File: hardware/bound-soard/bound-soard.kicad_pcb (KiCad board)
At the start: 2 copper layers, 17 parts, among them J1 Signal_Input, J2 Conn_01x02_Female, J3 Conn_01x02_Male, J4 Conn_01x02_Female, J5 Supply, J6 Conn_01x02_Male, J7 Conn_01x02_Female, J8 Conn_01x02_Male, J9 Signal_Output

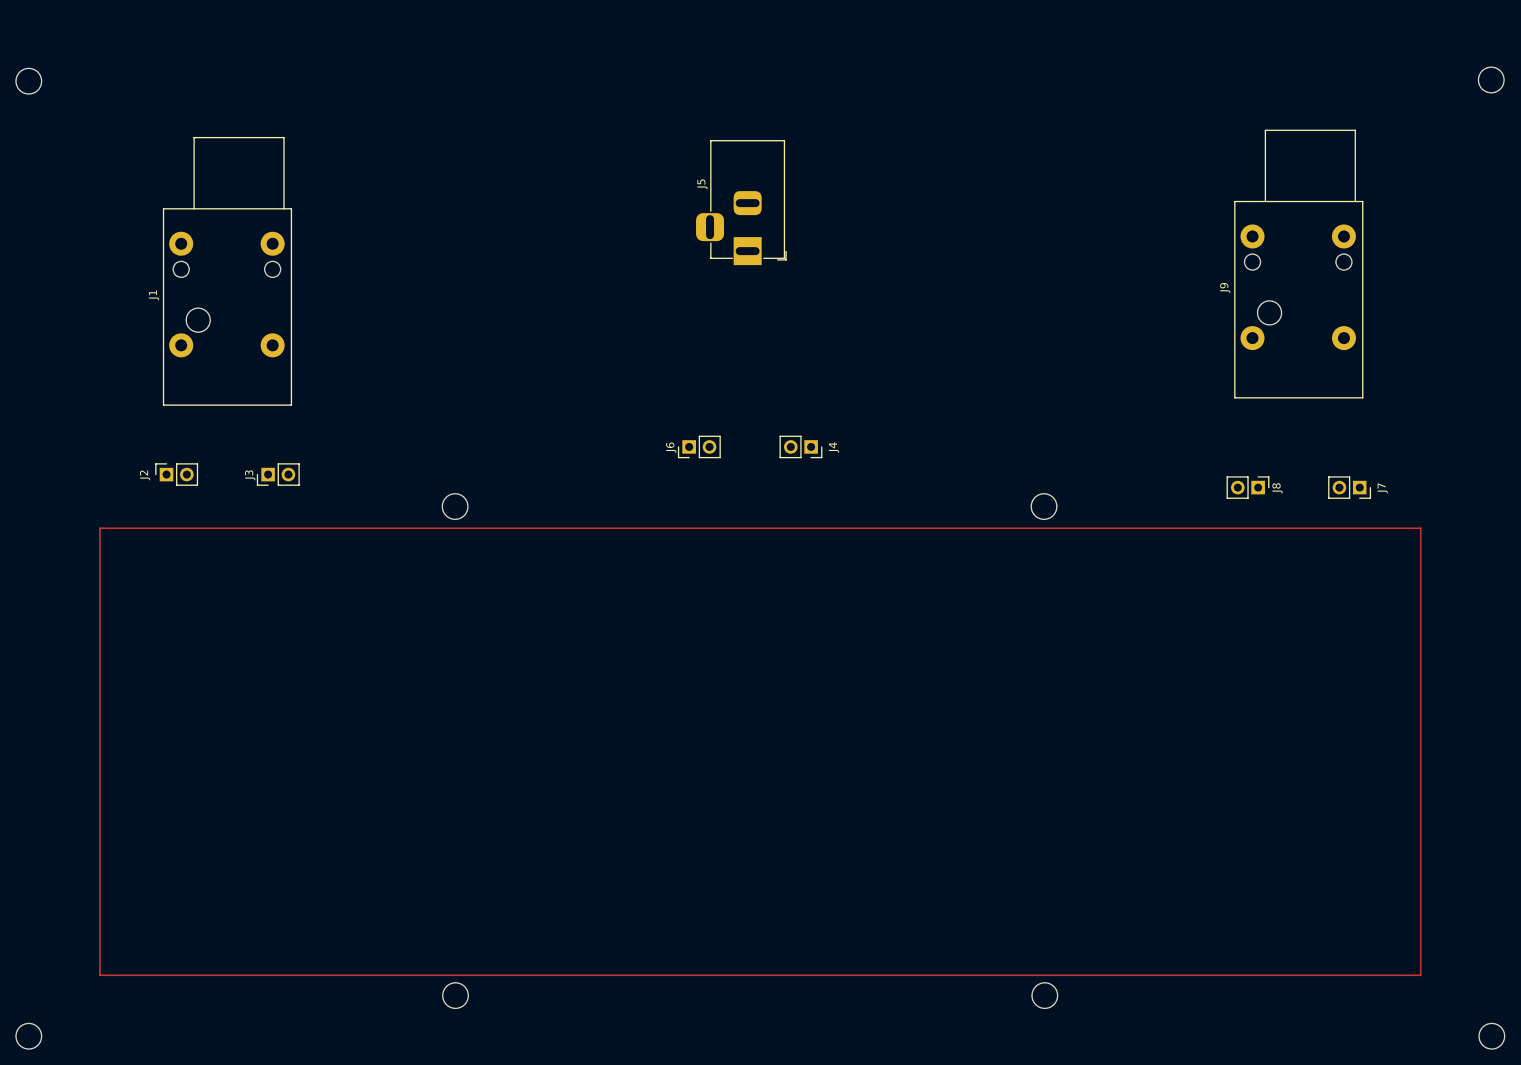
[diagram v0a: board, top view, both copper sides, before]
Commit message: probably final
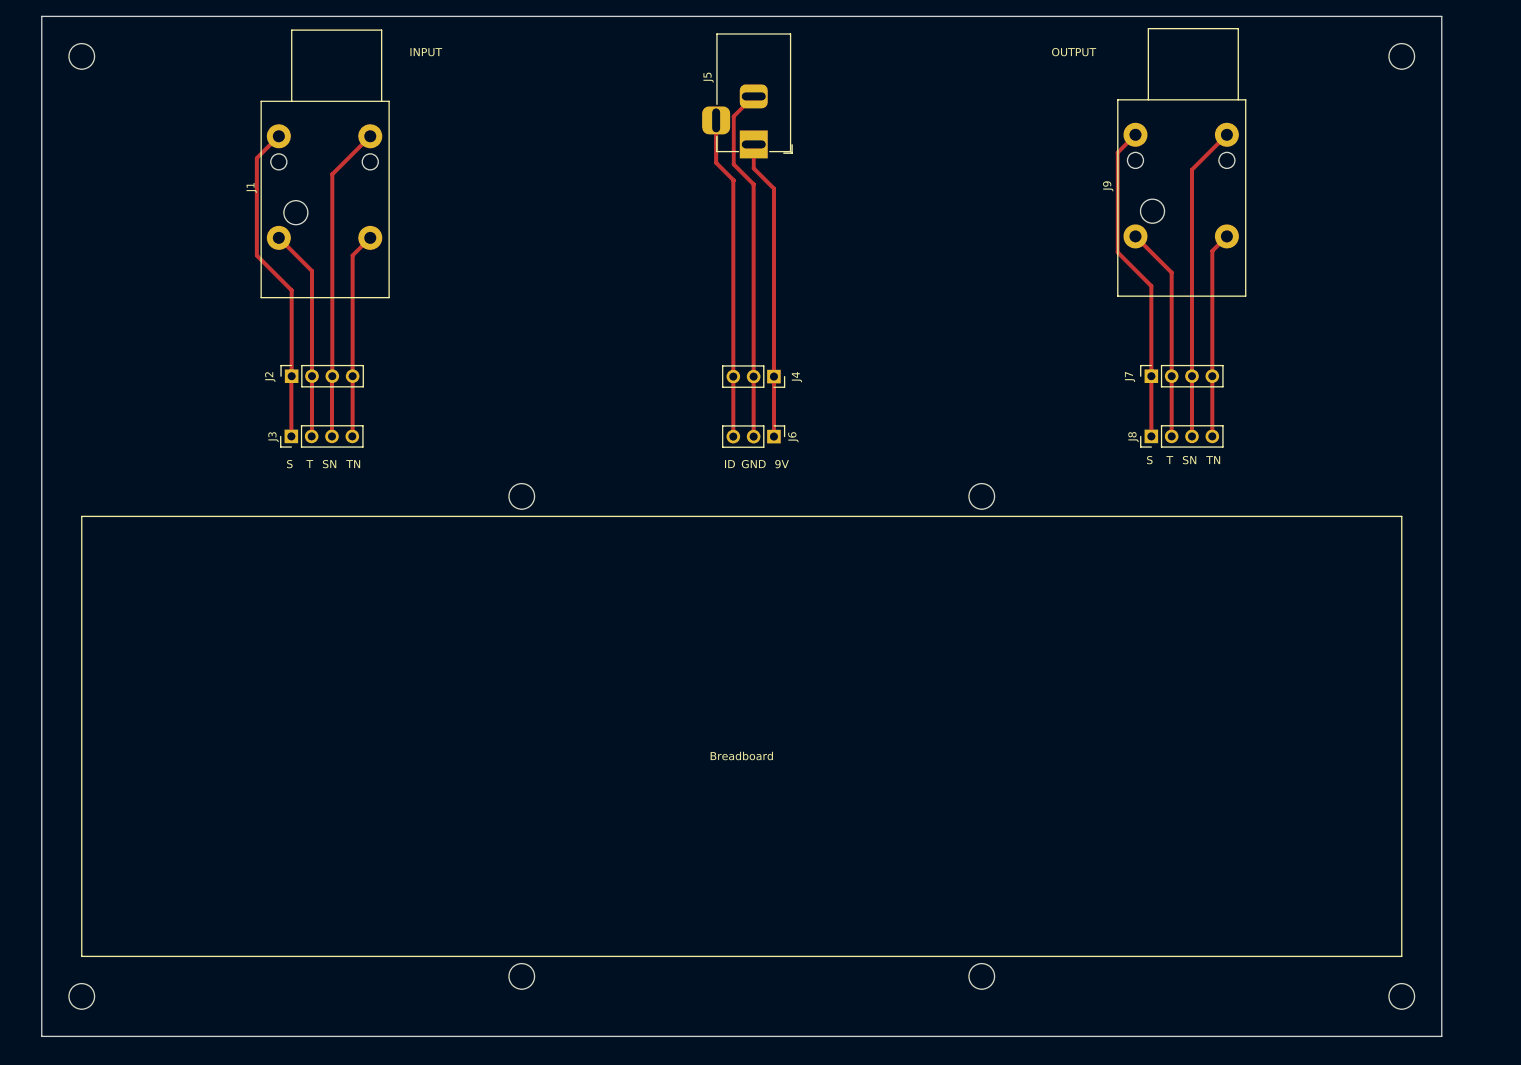
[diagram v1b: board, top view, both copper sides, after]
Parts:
- removed the REF** at (55.9, 38.1)
- removed the REF** at (238.7, 37.9)
- removed the REF** at (182.9, 152.4)
- removed the REF** at (238.8, 157.5)
- removed the REF** at (182.8, 91.3)
- removed the REF** at (55.9, 157.5)
- removed the REF** at (109.2, 152.4)
- removed the REF** at (109.2, 91.3)
- added REF**: MountingHole_3.2mm_M3_ISO14580, MountingHole:MountingHole_3.2mm_M3_ISO14580, F.Cu at (227.5, 152.5)
- added REF**: MountingHole_3.2mm_M3_ISO14580, MountingHole:MountingHole_3.2mm_M3_ISO14580, F.Cu at (117.5, 150.0)
- added REF**: MountingHole_3.2mm_M3_ISO14580, MountingHole:MountingHole_3.2mm_M3_ISO14580, F.Cu at (117.5, 90.0)
- added REF**: MountingHole_3.2mm_M3_ISO14580, MountingHole:MountingHole_3.2mm_M3_ISO14580, F.Cu at (62.5, 35.0)
- added REF**: MountingHole_3.2mm_M3_ISO14580, MountingHole:MountingHole_3.2mm_M3_ISO14580, F.Cu at (175.0, 90.0)
- added REF**: MountingHole_3.2mm_M3_ISO14580, MountingHole:MountingHole_3.2mm_M3_ISO14580, F.Cu at (62.5, 152.5)
- added REF**: MountingHole_3.2mm_M3_ISO14580, MountingHole:MountingHole_3.2mm_M3_ISO14580, F.Cu at (175.0, 150.0)
- added REF**: MountingHole_3.2mm_M3_ISO14580, MountingHole:MountingHole_3.2mm_M3_ISO14580, F.Cu at (227.5, 35.0)
- J1: value Signal_Input -> AudioJack2_Dual_Switch
- J2, J7: value Conn_01x02_Female -> Conn_01x04_Female; footprint Connector_PinSocket_2.54mm:PinSocket_1x02_P2.54mm_Vertical -> Connector_PinSocket_2.54mm:PinSocket_1x04_P2.54mm_Vertical
- J3, J8: value Conn_01x02_Male -> Conn_01x04_Male; footprint Connector_PinHeader_2.54mm:PinHeader_1x02_P2.54mm_Vertical -> Connector_PinHeader_2.54mm:PinHeader_1x04_P2.54mm_Vertical
- J4: value Conn_01x02_Female -> Conn_01x03_Female; footprint Connector_PinSocket_2.54mm:PinSocket_1x02_P2.54mm_Vertical -> Connector_PinSocket_2.54mm:PinSocket_1x03_P2.54mm_Vertical
- J5: value Supply -> 9V Supply
- J6: value Conn_01x02_Male -> Conn_01x03_Male; footprint Connector_PinHeader_2.54mm:PinHeader_1x02_P2.54mm_Vertical -> Connector_PinHeader_2.54mm:PinHeader_1x03_P2.54mm_Vertical
- J9: value Signal_Output -> AudioJack2_Dual_Switch
- moved J7 29.5 mm to (196.2, 75.0), turned to 90 degrees
- moved J2 19.9 mm to (88.7, 75.0)
- moved J9 19.4 mm to (194.2, 57.5)
- moved J1 18.2 mm to (87.1, 57.7)
- moved J8 14.8 mm to (196.2, 82.5), turned to 90 degrees
- moved J5 13.4 mm to (146.5, 46.0)
- moved J6 10.7 mm to (149.0, 82.5), turned to -90 degrees
- moved J4 9.95 mm to (149.0, 75.0)
- moved J3 5.58 mm to (88.7, 82.5)
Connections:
- J1 pad SN: (no net) -> Net-(J1-PadSN)
- J1 pad TN: (no net) -> Net-(J1-PadTN)
- J5 pad 3: (no net) -> Net-(J4-Pad3)
- J9 pad SN: (no net) -> Net-(J7-Pad3)
- J9 pad TN: (no net) -> Net-(J7-Pad4)
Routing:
- net Net-(J4-Pad2): track 0.00 -> 44.6 mm
- net Net-(J4-Pad3): track 0.00 -> 41.4 mm
- net Net-(J1-PadS): track 0.00 -> 40.5 mm
- net Net-(J7-Pad1): track 0.00 -> 40.3 mm
- net Net-(J1-PadSN): track 0.00 -> 39.8 mm
- net Net-(J7-Pad3): track 0.00 -> 39.5 mm
- net Net-(J4-Pad1): track 0.00 -> 37.6 mm
- net Net-(J7-Pad2): track 0.00 -> 26.8 mm
- net Net-(J1-PadT): track 0.00 -> 26.6 mm
- net Net-(J1-PadTN): track 0.00 -> 25.8 mm
- net Net-(J7-Pad4): track 0.00 -> 25.7 mm
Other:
- board outline added: 175 x 127.5 mm
- board text added: "9V"
- board text added: "Breadboard"
- board text added: "GND"
- board text added: "ID"
- board text added: "INPUT"
- board text added: "OUTPUT"
- board text added: "S"
- board text added: "SN"
- board text added: "T"
- board text added: "TN"
